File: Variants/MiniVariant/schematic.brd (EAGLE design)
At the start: 87 x 58 mm, 12 parts, among them U1 TMP75_D_8, U2 SHT21

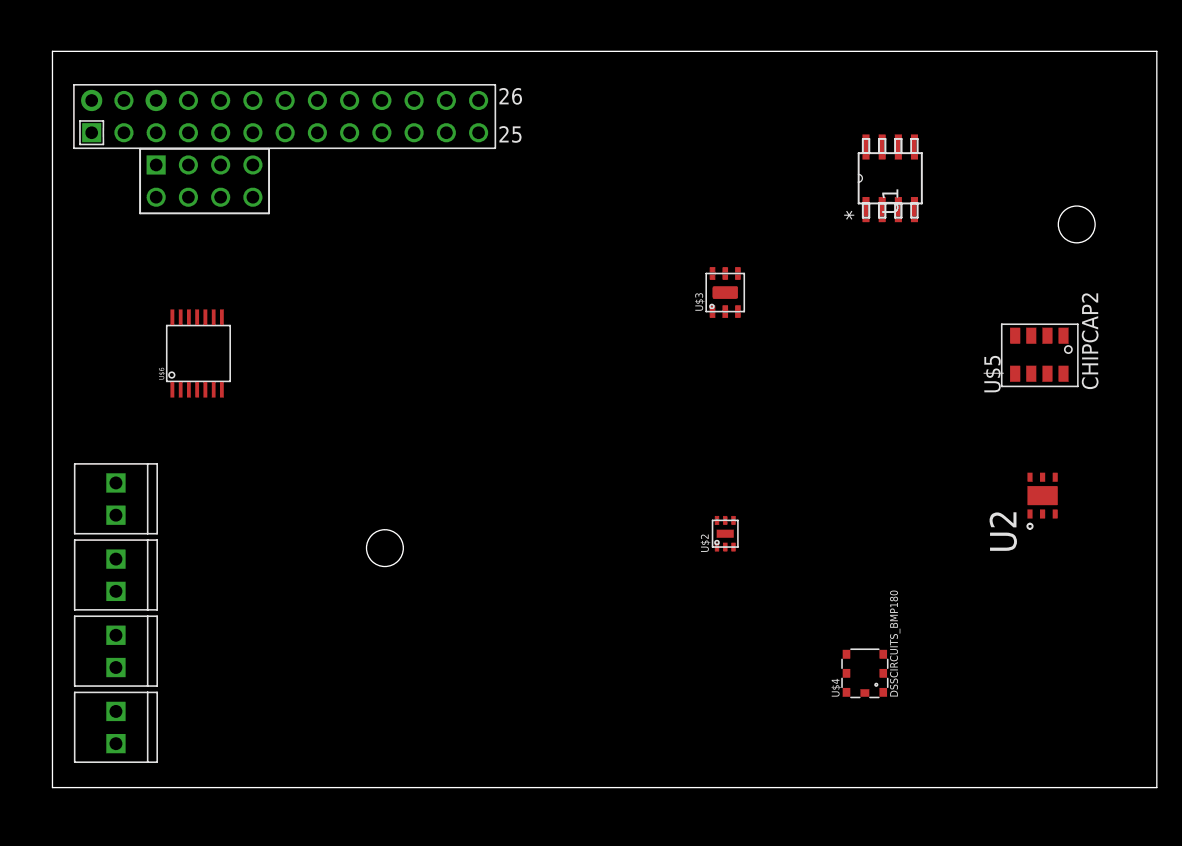
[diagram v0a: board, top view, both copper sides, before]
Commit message: Normal Push
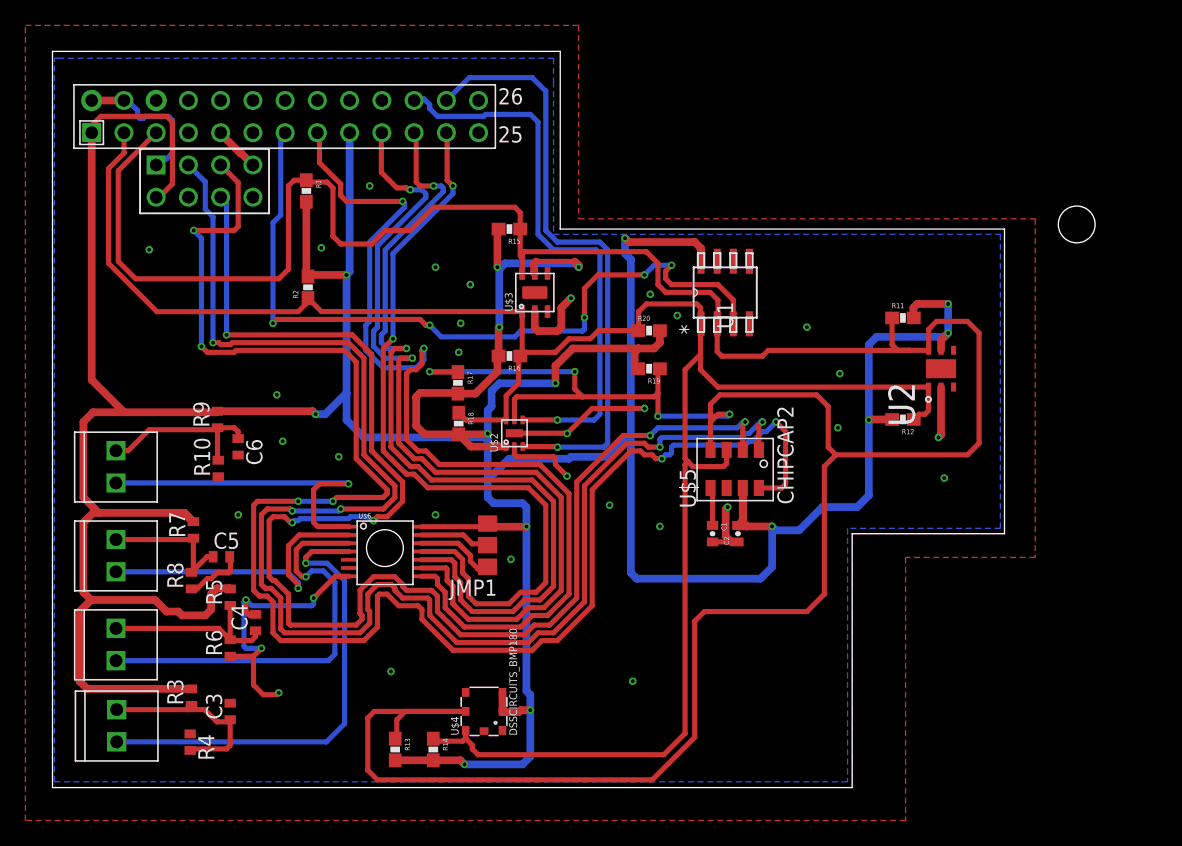
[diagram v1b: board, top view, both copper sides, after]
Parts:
- added C1: 100nF, weatherpilot_lbr:0402-CAP
- added C2: 220nF, weatherpilot_lbr:0402-CAP
- added C3, C4, C5, C6: (no value), rcl:C0402
- added JMP1: 0R-JUMPA, jump-0r-smd:A0R-JMP
- added R1, R11, R12, R13, R14, R15, R16, R17, R18, R19, R2, R20: 10k, SparkFun-Resistors:0603-RES
- added R10, R3, R4, R5, R6, R7, R8, R9: (no value), rcl:R0402
- U$1: device lib:RASPBERRY-PI_REV2 -> RaspberryPi:RASPBERRY-PI_REV2
- moved U$4 30.1 mm to (34.0, 6.00)
- moved U$5 25.6 mm to (54.0, 25.0)
- moved U$6 18.9 mm to (24.0, 16.0), turned to 0 degrees
- moved U$2 18.4 mm to (36.4, 27.9)
- moved U1 15.8 mm to (53.0, 39.0)
- moved U$3 15.0 mm to (38.0, 39.0)
- moved JP1 14.0 mm to (5.00, 10.0), turned to 90 degrees
- moved U2 12.8 mm to (70.0, 33.0)
- moved JP3 12.0 mm to (5.00, 24.0), turned to 90 degrees
- moved JP4 2.40 mm to (5.06, 3.60), turned to 90 degrees
- moved JP2 1.00 mm to (5.00, 17.0), turned to 90 degrees
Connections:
- removed net V+: U1.8
- removed net VDD: U$4.2, U2.5
- removed net VDDIO: U$4.3
- removed net VSS: U2.2
- new net +3V3: C2.2, JMP1.3, R1.2, R11.2, R12.2, R13.2, R14.2, R15.2, R16.2, R17.2, R18.2, R19.2, R2.2, R20.2, R3.2, R5.2, R7.2, R9.2, U$1.P1_1, U$1.P1_17, U$1.P5_2, U$2.P1, U$3.VDD, U$4.2, U$4.3, U$5.7, U$6.P$14, U1.8, U2.5
- new net ALARM_HIGH: U$1.P5_5, U$5.8
- new net ALARM_LOW: U$1.P5_3, U$5.1
- new net CH0: JP3.P2, U$6.P$1
- new net CH1: JP2.P2, U$6.P$2
- new net CH2: JP1.P2, U$6.P$3
- new net CH3: JP4.P2, U$6.P$4
- new net GPIO25: U$1.P1_22, U$2.P4
- new net GPIO8: U$1.P1_24, U$2.P3
- new net MISO: U$1.P1_21, U$6.P$10
- new net MOSI: U$1.P1_19, U$6.P$9
- new net N$1: C4.1, JP1.P1, R5.1, R6.2
- new net N$12: C3.1, JP4.P1, R3.1, R4.2
- new net N$17: JMP1.2, U$6.P$13
- new net N$2: C5.1, JP2.P1, R7.1, R8.2
- new net N$3: U$1.P5_4
- new net N$4: C6.1, JP3.P1, R10.2, R9.1
- new net N$5: C1.1, U$5.5
- new net READY: U$1.P5_6, U$5.2
- new net SCK: U$1.P1_23, U$6.P$11
- new net SCL: R1.1, R11.1, R13.1, R15.1, R17.1, R19.1, U$1.P1_5, U$2.P5, U$3.SCL, U$4.5, U$5.4, U1.2, U2.6
- new net SDA: R12.1, R14.1, R16.1, R18.1, R2.1, R20.1, U$1.P1_3, U$2.P6, U$3.SDA, U$4.6, U$5.3, U1.1, U2.1
- new net SS: U$1.P1_15, U$6.P$8
- new net TMP_ALERT: U$1.P1_13, U1.3
- new net VCC: U$1.P1_2, U$1.P1_4, U$1.P5_1
- net GND: now also C1.2, C2.1, C3.2, C4.2, C5.2, C6.2, JMP1.1, R10.1, R4.1, R6.1, R8.1, U$1.P1_14, U$1.P1_20, U$1.P1_25, U$1.P1_6, U$1.P1_9, U$1.P5_7, U$1.P5_8, U$2.P2, U$2.PAD, U$3.GND, U$3.T_GND, U$5.6, U$6.P$12, U$6.P$7, U1.5, U1.6, U1.7, U2.2, U2.7
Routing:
- net +3V3: track 0.00 -> 378.9 mm, vias 0 -> 15
- net SCL: track 0.00 -> 267.1 mm, vias 0 -> 4
- net SDA: track 0.00 -> 160.3 mm
- net ALARM_HIGH: track 0.00 -> 130.7 mm, vias 0 -> 6
- net ALARM_LOW: track 0.00 -> 119.8 mm, vias 0 -> 5
- net READY: track 0.00 -> 112.7 mm, vias 0 -> 5
- net SS: track 0.00 -> 76.0 mm, vias 0 -> 2
- net GND: track 0.00 -> 71.3 mm, vias 0 -> 33
- net MOSI: track 0.00 -> 69.1 mm, vias 0 -> 2
- net MISO: track 0.00 -> 67.1 mm, vias 0 -> 2
- net SCK: track 0.00 -> 61.9 mm, vias 0 -> 2
- net TMP_ALERT: track 0.00 -> 60.9 mm, vias 0 -> 5
- net GPIO8: track 0.00 -> 47.6 mm, vias 0 -> 1
- net GPIO25: track 0.00 -> 44.2 mm, vias 0 -> 1
- net CH3: track 0.00 -> 37.5 mm, vias 0 -> 1
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- added copper zone on layer 1, net GND
- added copper zone on layer 16, net GND
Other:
- board size 87 x 58 mm -> 75 x 58 mm
